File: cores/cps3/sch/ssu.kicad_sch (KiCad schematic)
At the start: 1 part

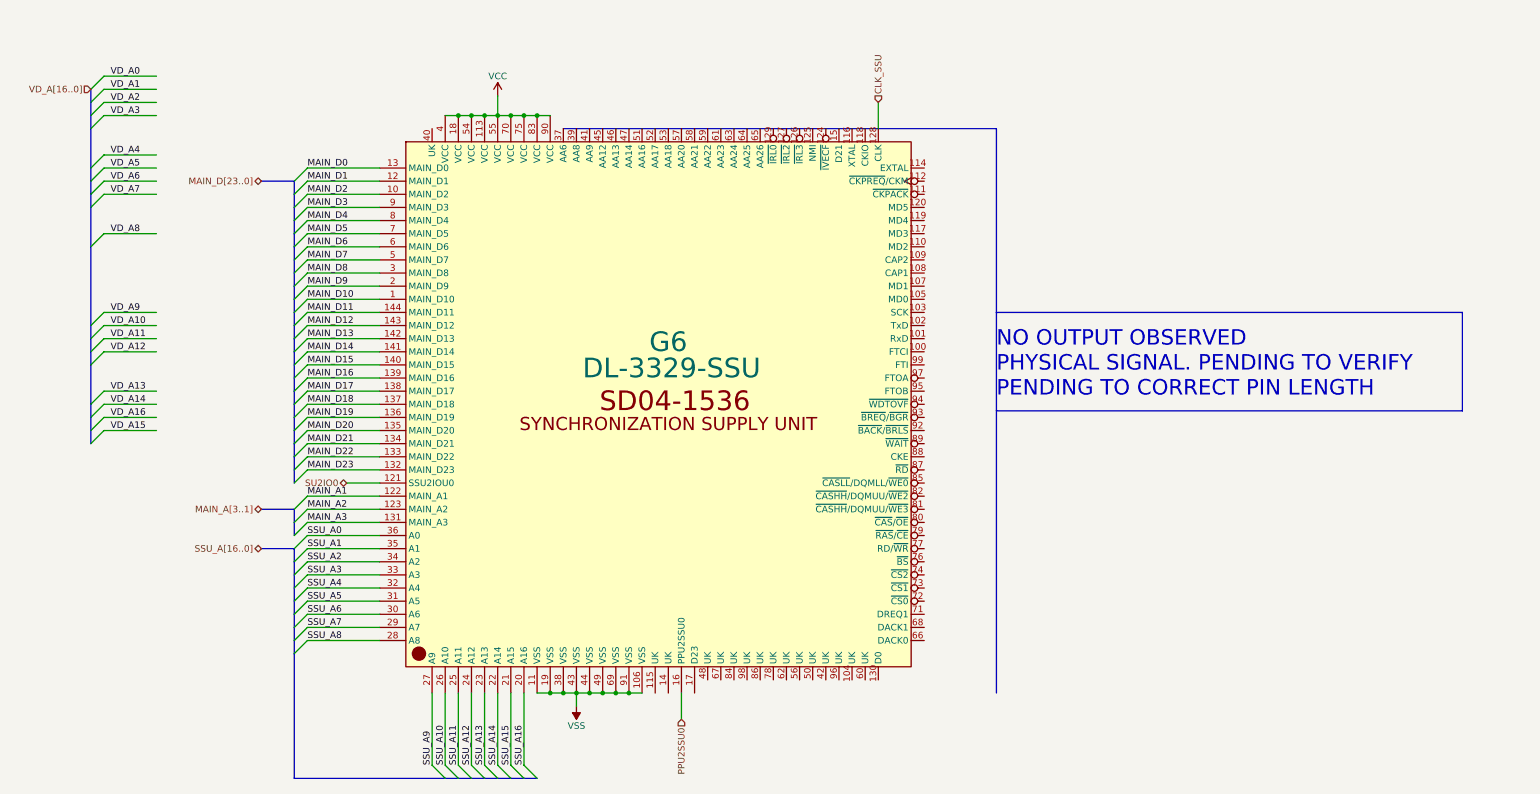
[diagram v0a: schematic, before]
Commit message: wip_ssu_cbi_gll
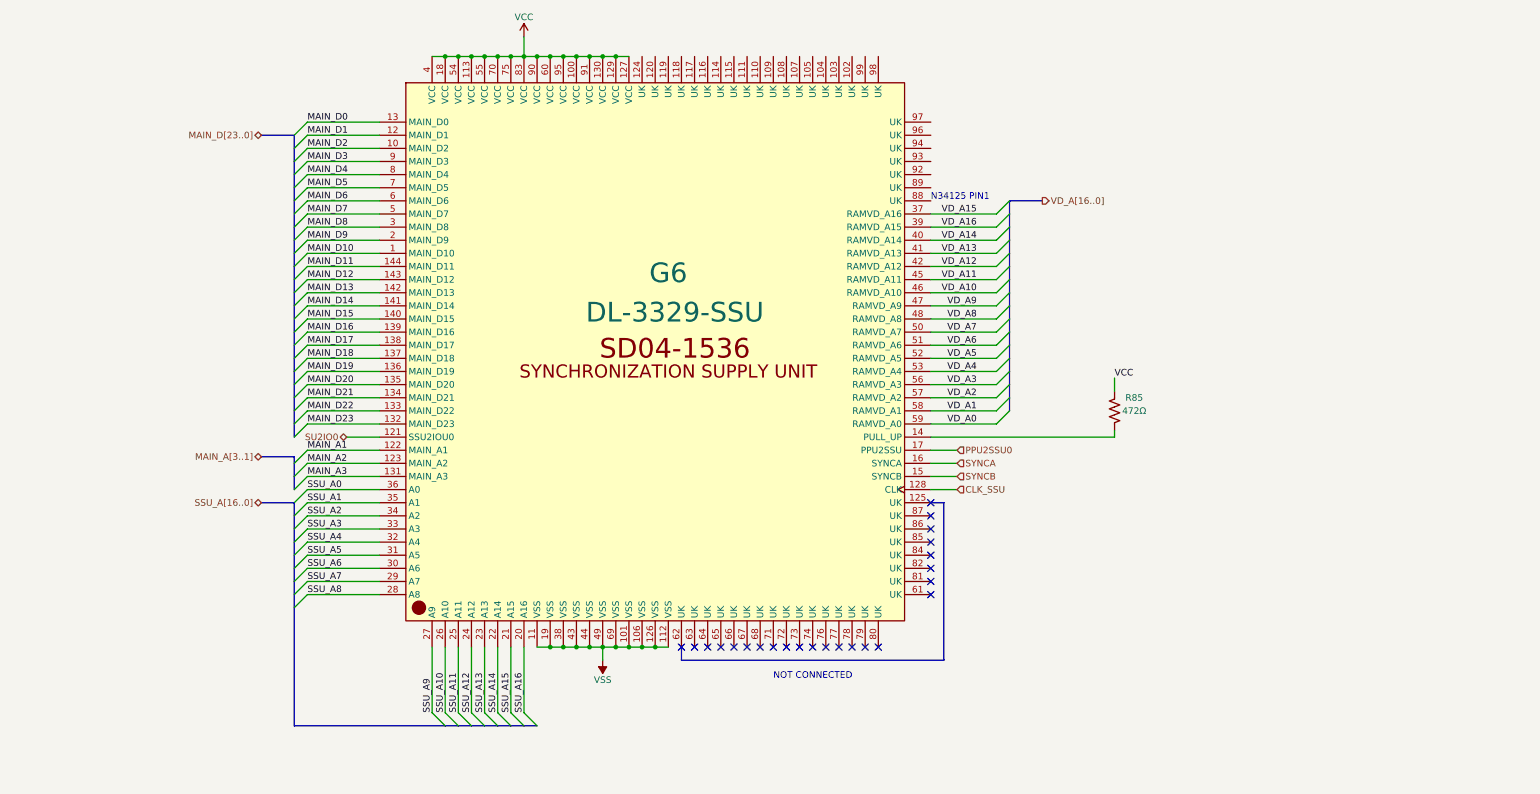
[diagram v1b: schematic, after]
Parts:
- added R85: 472Ω, symbol Device:R_US
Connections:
- net PPU2SSU0: now also G6.17 (PPU2SSU); no longer G6.16 (PPU2SSU0)
- net VCC: now also G6.100 (VCC), G6.127 (VCC), G6.129 (VCC), G6.130 (VCC), G6.60 (VCC), G6.91 (VCC), G6.95 (VCC), R85.2
- net VD_A0: now also G6.59 (RAMVD_A0)
- net VD_A1: now also G6.58 (RAMVD_A1)
- net VD_A10: now also G6.46 (RAMVD_A10)
- net VD_A11: now also G6.45 (RAMVD_A11)
- net VD_A12: now also G6.42 (RAMVD_A12)
- net VD_A13: now also G6.41 (RAMVD_A13)
- net VD_A14: now also G6.40 (RAMVD_A14)
- net VD_A15: now also G6.37 (RAMVD_A16)
- net VD_A16: now also G6.39 (RAMVD_A15)
- net VD_A2: now also G6.57 (RAMVD_A2)
- net VD_A3: now also G6.56 (RAMVD_A3)
- net VD_A4: now also G6.53 (RAMVD_A4)
- net VD_A5: now also G6.52 (RAMVD_A5)
- net VD_A6: now also G6.51 (RAMVD_A6)
- net VD_A7: now also G6.50 (RAMVD_A7)
- net VD_A8: now also G6.48 (RAMVD_A8)
- net VD_A9: now also G6.47 (RAMVD_A9)
- net VSS: now also G6.101 (VSS), G6.112 (VSS), G6.126 (VSS); no longer G6.91 (VSS)
- net at G6.14 (PULL_UP): now also R85.1
- net SYNCB: now reaches G6.15 (SYNCB)
- new net SYNCA: G6.16 (SYNCA)
- no-connect marks 0 -> 24
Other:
- note added: "N34125 PIN1"
- note added: "NOT CONNECTED"
- note removed: "NO OUTPUT OBSERVED PHYSICAL SIGNAL. PENDING TO VERIFY PENDING TO CORRECT PIN LENGTH"
